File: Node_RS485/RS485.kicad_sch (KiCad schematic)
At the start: 16 parts, among them J2 CONN_RS485, U2 SP3485EN

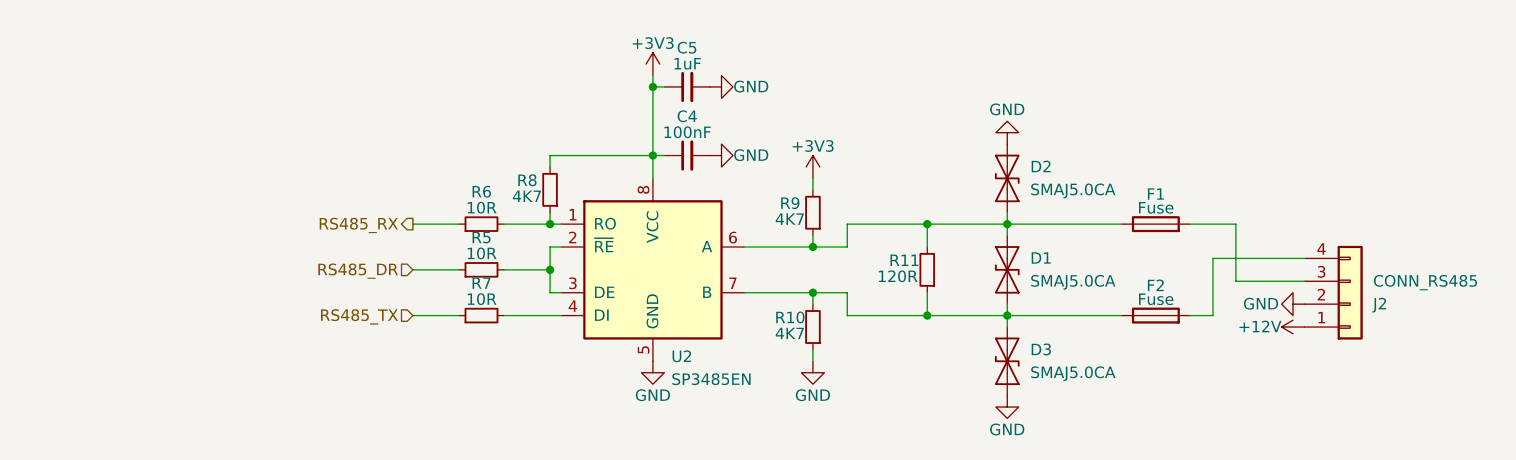
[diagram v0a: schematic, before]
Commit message: New version.
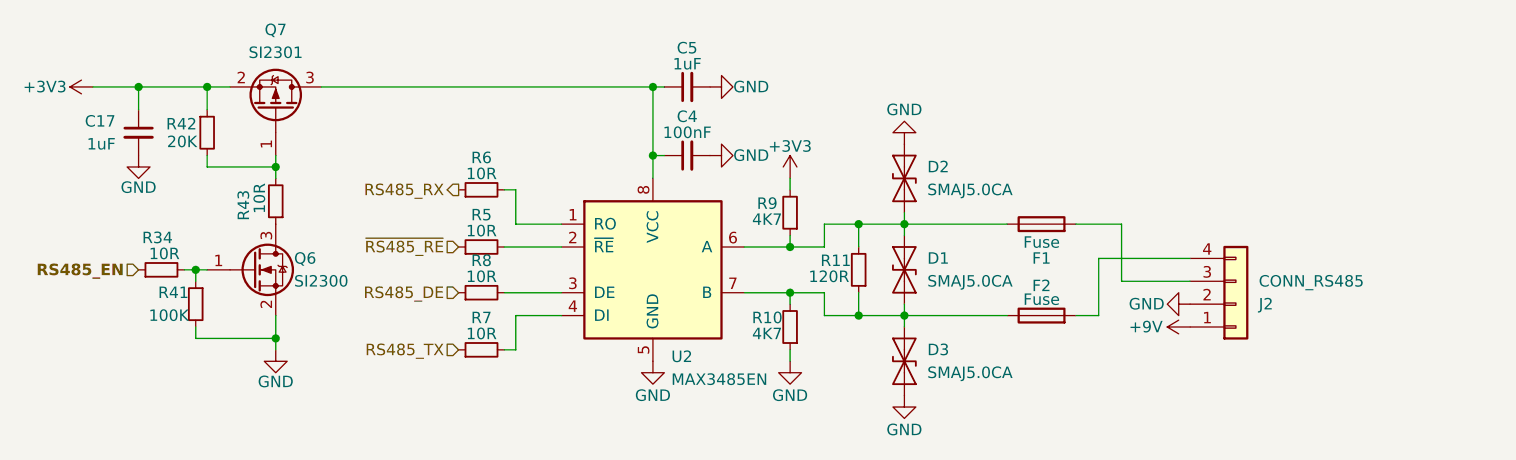
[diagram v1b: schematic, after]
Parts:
- added C17: 1uF, Footprints:C_0603, symbol Device:C_Small
- added Q6: SI2300, Footprints:SOT23-3, symbol Transistor_FET:2N7002
- added Q7: SI2301, Footprints:SOT23-3, symbol Transistor_FET:AO3401A
- added R34, R43: 10R, Footprints:R_0603, symbol Device:R_Small
- added R41: 100K, Footprints:R_0603, symbol Device:R_Small
- added R42: 20K, Footprints:R_0603, symbol Device:R_Small
- R8: value 4K7 -> 10R
- U2: value SP3485EN -> MAX3485EN
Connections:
- net +3V3: now also C17.1, Q7.2 (S), R42.1; no longer C4.1, C5.1, R8.2, U2.8 (VCC)
- net GND: now also C17.2, Q6.2 (S), R41.2
- net at R5.2, U2.2 (~{RE}): no longer U2.3 (DE)
- net at R6.2, U2.1 (RO): no longer R8.1
- net +12V renamed +9V
- net RS485_DR renamed ~{RS485_RE}
- new net: Q7.1 (G), R42.2, R43.2
- new net: Q6.1 (G), R34.2, R41.1
- new net: R8.2, U2.3 (DE)
- new net: Q6.3 (D), R43.1
- new net: C4.1, C5.1, Q7.3 (D), U2.8 (VCC)
- new net RS485_DE: R8.1
- new net RS485_EN: R34.1
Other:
- moved on the sheet: D1, D2, D3, F1, F2, J2, R10, R11, R5, R6, R7, R9
